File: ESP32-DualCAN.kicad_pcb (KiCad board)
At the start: 2 copper layers, 19.6 x 38.8 mm, 28 parts, among them J1 Molex 70553 6p, J2 Conn_01x10_Socket, J3 Conn_01x10_Socket, J4 holes, J5 pads, J6 holes, J7 pads, U1 LV2862Y, U2 ESP32-C6-SuperMini, U3 TCAN1044AV, U4 TCAN1044AV

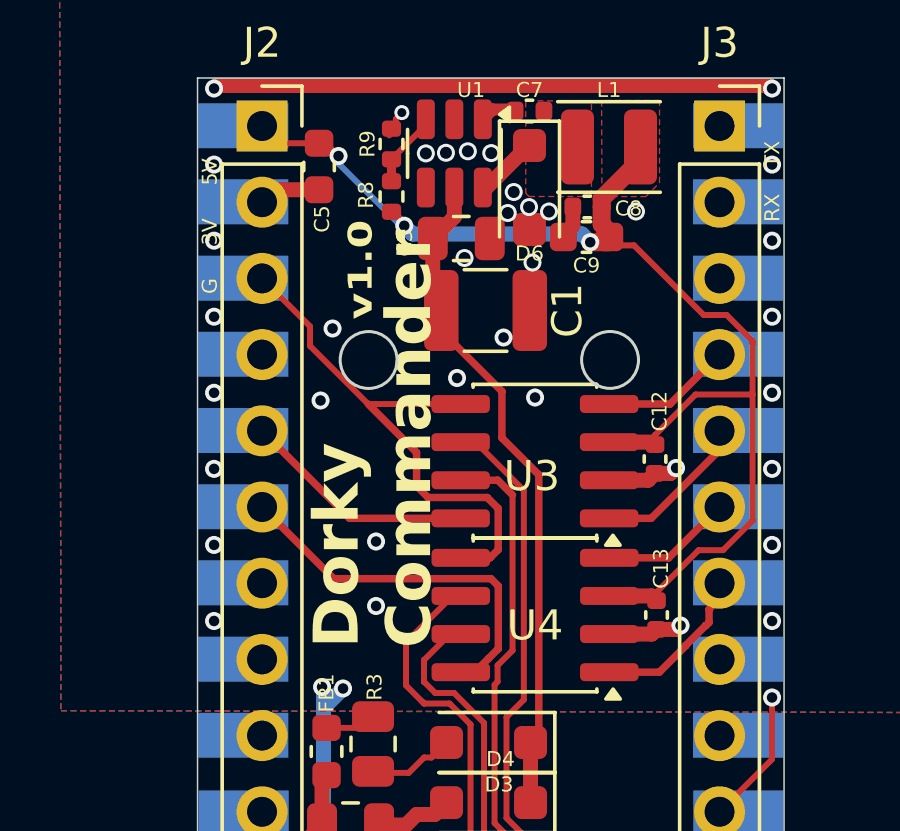
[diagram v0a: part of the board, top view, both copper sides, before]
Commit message: cleanup
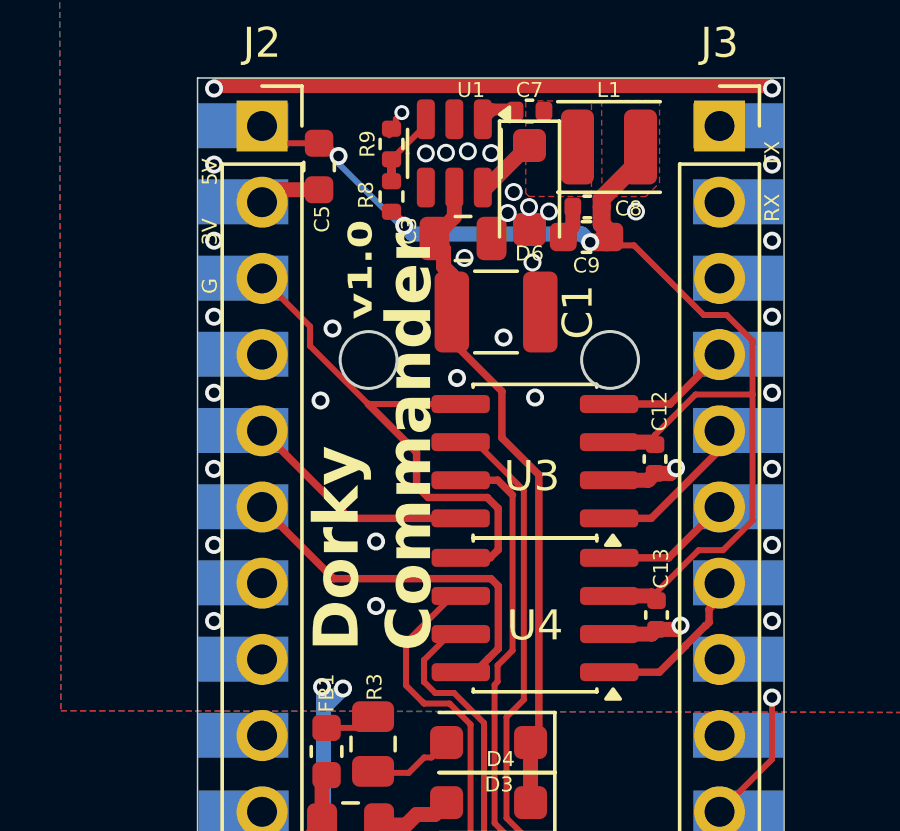
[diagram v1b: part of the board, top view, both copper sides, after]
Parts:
- moved C1 0.35 mm to (129.4, 87.0)
- moved C3 0.06 mm to (128.3, 84.6)

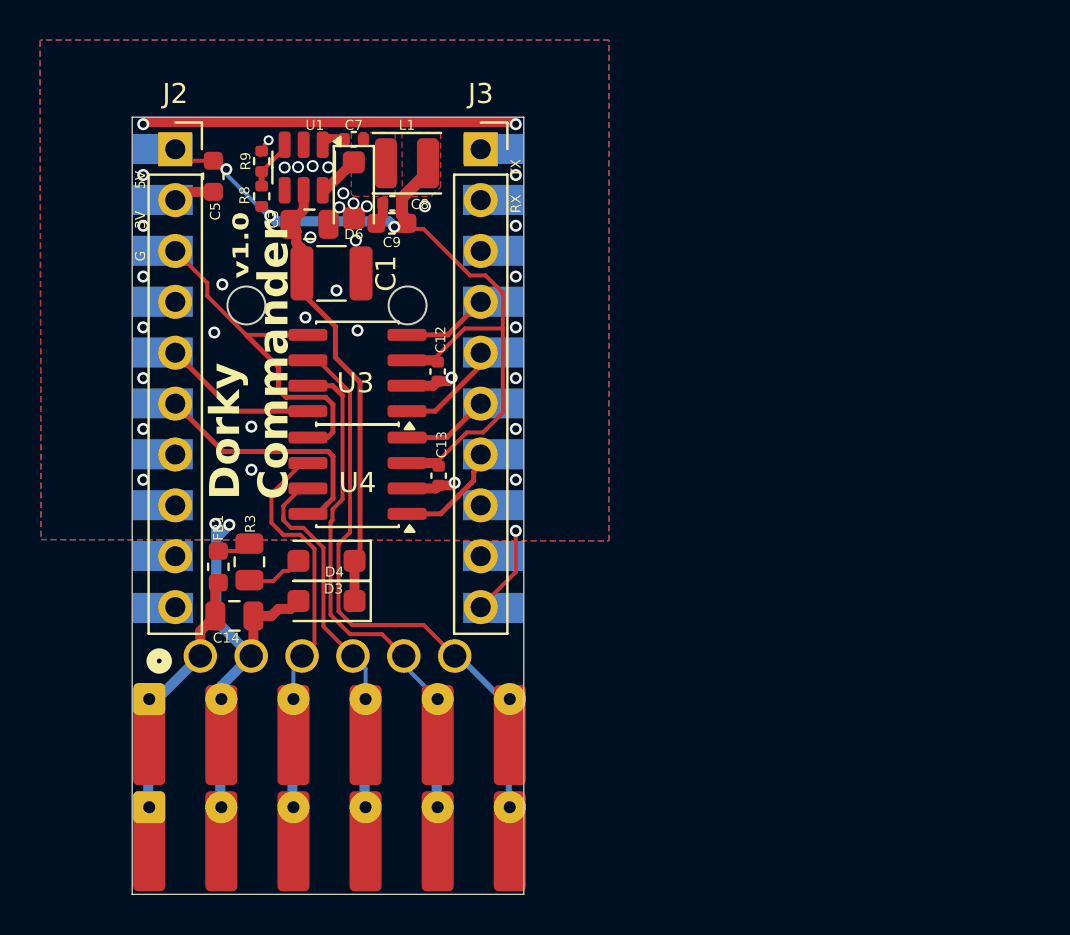
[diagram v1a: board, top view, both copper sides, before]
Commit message: horizontal layout
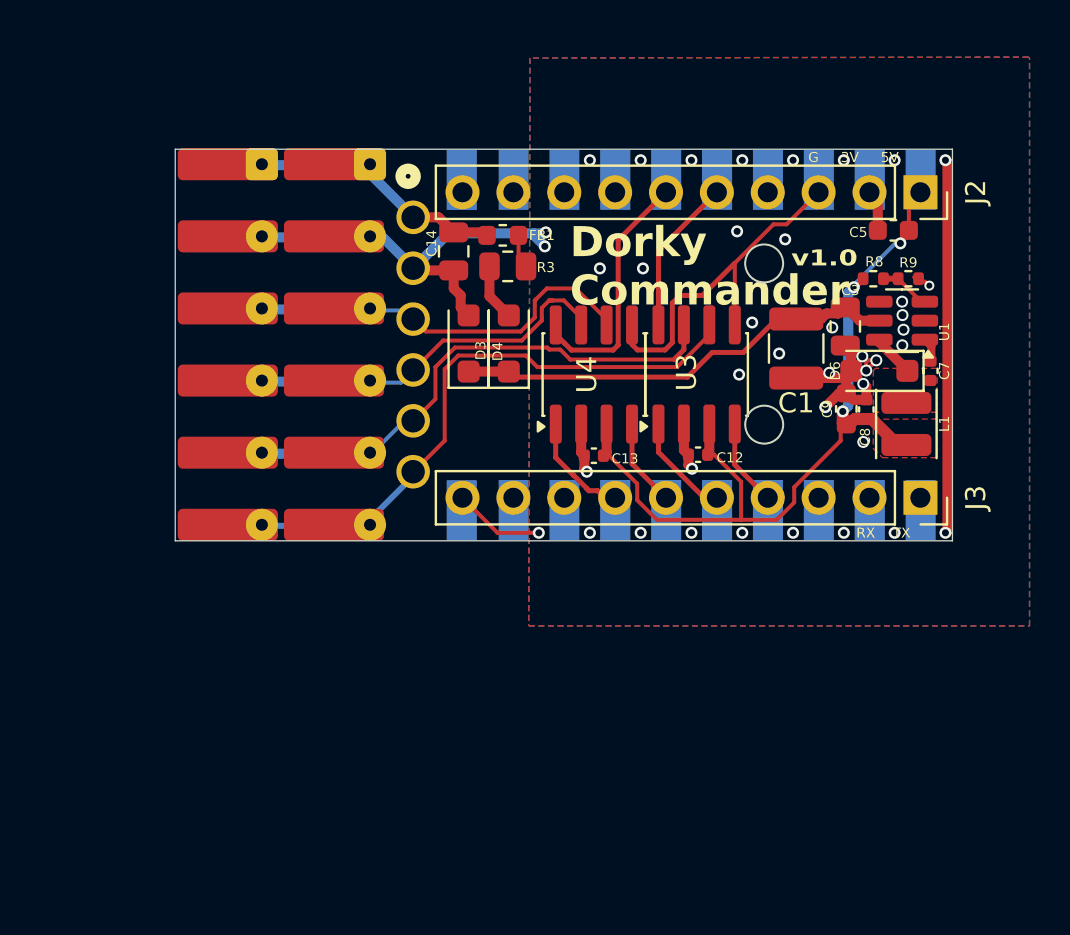
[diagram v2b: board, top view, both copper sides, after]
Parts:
- moved J2 37.3 mm to (158.8, 83.0), turned to -90 degrees
- moved C5 34.1 mm to (157.5, 84.9), turned to 180 degrees
- moved J7 34.0 mm to (124.3, 81.6), turned to -90 degrees
- moved R9 32.8 mm to (158.2, 87.3), turned to 180 degrees
- moved J4 32.6 mm to (126.0, 81.6), turned to -90 degrees
- moved C7 31.0 mm to (159.3, 91.9), turned to -90 degrees
- moved U1 30.8 mm to (157.9, 89.4), turned to 180 degrees
- moved R8 30.8 mm to (156.5, 87.3), turned to 180 degrees
- moved J5 30.0 mm to (129.6, 81.6), turned to -90 degrees
- moved J6 28.9 mm to (131.4, 81.6), turned to -90 degrees
- moved L1 28.1 mm to (158.2, 94.6), turned to -90 degrees
- moved J3 28.0 mm to (158.8, 98.2), turned to -90 degrees
- moved D6 27.7 mm to (156.8, 91.9), turned to 180 degrees
- moved C3 27.2 mm to (155.1, 89.7), turned to -90 degrees
- moved C8 25.8 mm to (156.2, 93.8), turned to 90 degrees
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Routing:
- net GND: track 53.1 -> 63.1 mm, vias 40 -> 41
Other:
- board size 19.6 x 38.8 mm -> 38.8 x 19.6 mm
